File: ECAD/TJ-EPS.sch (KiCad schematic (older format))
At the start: 29 parts

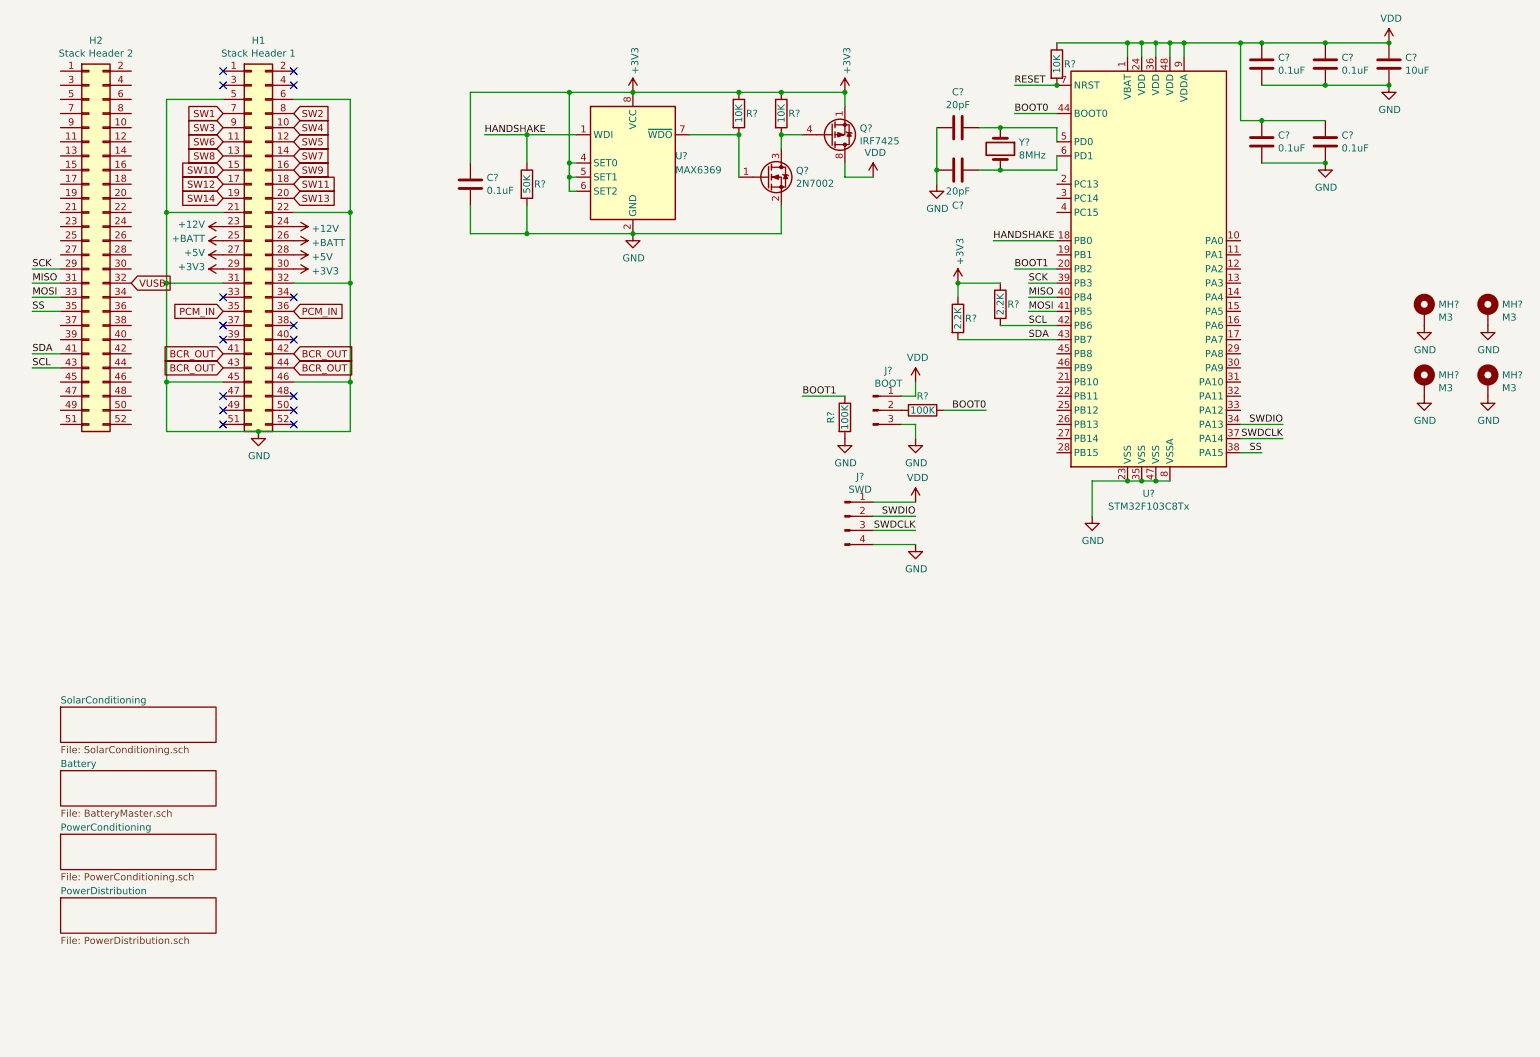
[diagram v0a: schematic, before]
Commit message: add amux
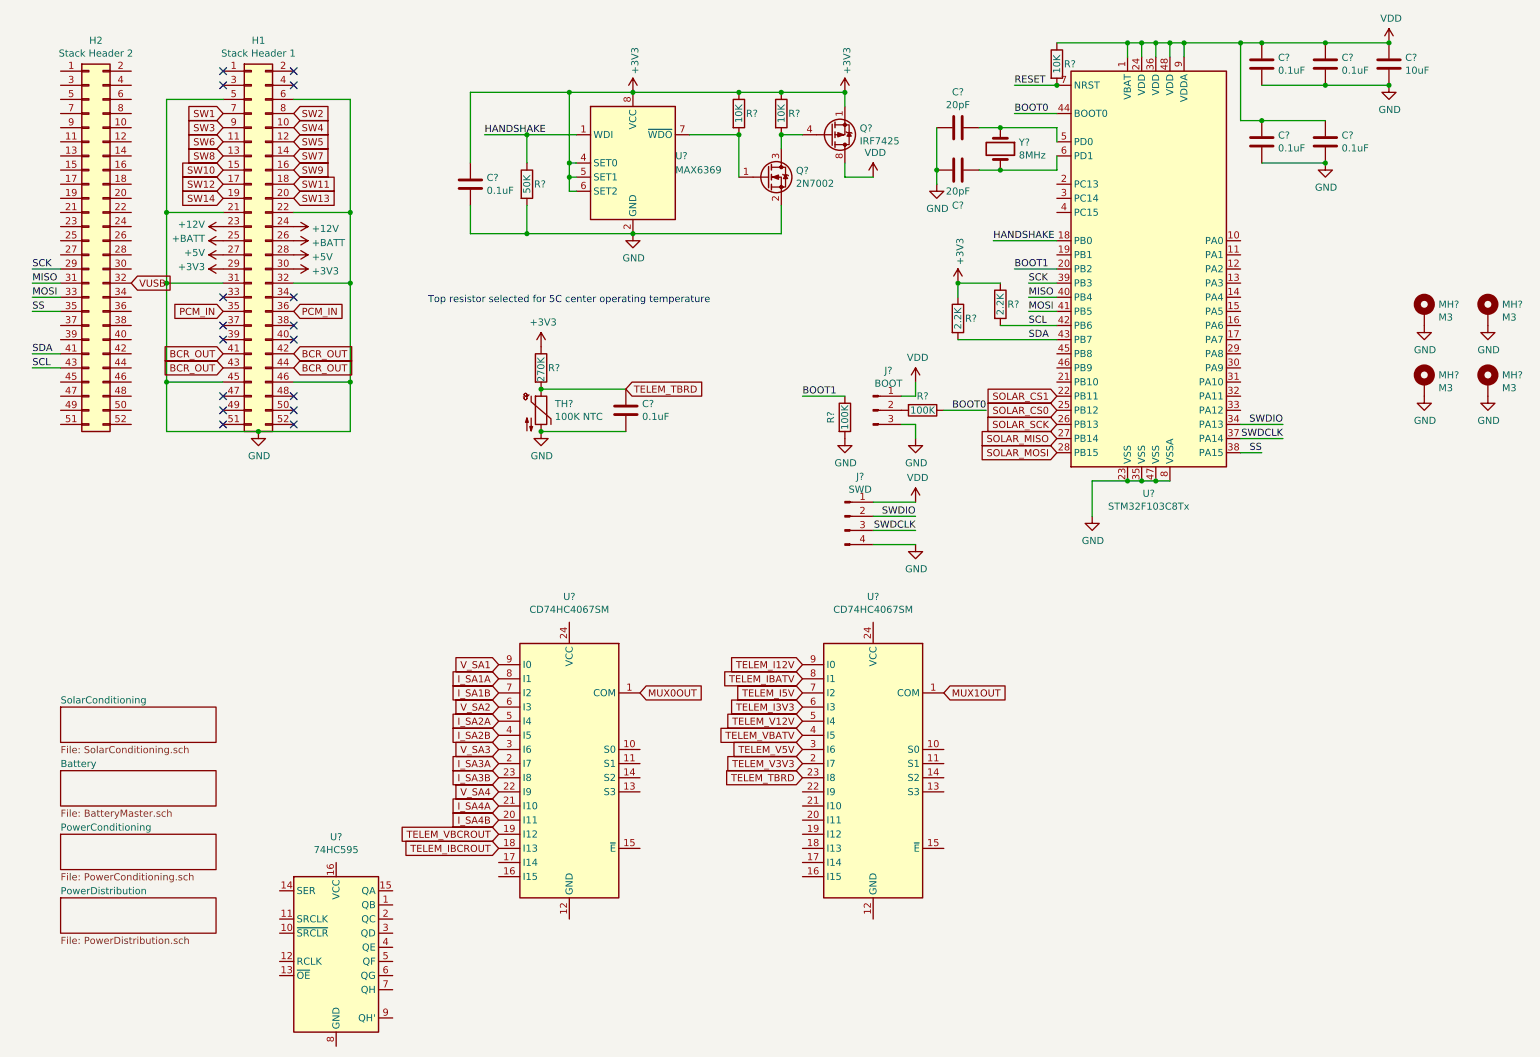
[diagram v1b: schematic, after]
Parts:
- added C?: 0.1uF, symbol Device:C
- added R?: 270K, symbol Device:R
- added TH?: 100K NTC, symbol Device:Thermistor_NTC
- added U? (x2): CD74HC4067SM, Package_SO:SSOP-24_5.3x8.2mm_P0.65mm, symbol 74xx:CD74HC4067SM
- added U?: 74HC595, symbol 74xx:74HC595
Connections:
- net +3V3: now also R?.1
- net GND: now also C?.2, TH?.2
- net SOLAR_CS1: now reaches U?.22 (PB11)
- net SOLAR_CS0: now reaches U?.25 (PB12)
- net SOLAR_SCK: now reaches U?.26 (PB13)
- net SOLAR_MISO: now reaches U?.27 (PB14)
- net SOLAR_MOSI: now reaches U?.28 (PB15)
- new net I_SA1A: U?.8 (I1)
- new net I_SA1B: U?.7 (I2)
- new net I_SA2A: U?.5 (I4)
- new net I_SA2B: U?.4 (I5)
- new net I_SA3A: U?.2 (I7)
- new net I_SA3B: U?.23 (I8)
- new net I_SA4A: U?.21 (I10)
- new net I_SA4B: U?.20 (I11)
- new net MUX0OUT: U?.1 (COM)
- new net MUX1OUT: U?.1 (COM)
- new net TELEM_I12V: U?.9 (I0)
- new net TELEM_I3V3: U?.6 (I3)
- new net TELEM_I5V: U?.7 (I2)
- new net TELEM_IBATV: U?.8 (I1)
- new net TELEM_IBCROUT: U?.18 (I13)
- new net TELEM_TBRD: C?.1, R?.2, TH?.1, U?.23 (I8)
- new net TELEM_V12V: U?.5 (I4)
- new net TELEM_V3V3: U?.2 (I7)
- new net TELEM_V5V: U?.3 (I6)
- new net TELEM_VBATV: U?.4 (I5)
- new net TELEM_VBCROUT: U?.19 (I12)
- new net V_SA1: U?.9 (I0)
- new net V_SA2: U?.6 (I3)
- new net V_SA3: U?.3 (I6)
- new net V_SA4: U?.22 (I9)
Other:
- note added: "Top resistor selected for 5C center operating temperature"
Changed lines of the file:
@@
 Wire Wire Line
 	550  3050 750  3050
+$Comp
+L 74xx:CD74HC4067SM U?
+U 1 1 61D924A0
+P 4350 5850
+F 0 "U?" H 4350 7031 50  0000 C CNN
+F 1 "CD74HC4067SM" H 4350 6940 50  0000 C CNN
+F 2 "Package_SO:SSOP-24_5.3x8.2mm_P0.65mm" H 5400 4850 50  0001 C CIN
+F 3 "http://www.ti.com/lit/ds/symlink/cd74hc4067.pdf" H 4000 6700 50  0001 C CNN
+	1    4350 5850
+	-1   0    0    -1
+$EndComp
+Text GLabel 3850 5250 0    50   Input ~ 0
+I_SA1A
+Text GLabel 3850 5550 0    50   Input ~ 0
+I_SA2A
+Text GLabel 3850 5650 0    50   Input ~ 0
+I_SA2B
+Text GLabel 3850 5850 0    50   Input ~ 0
+I_SA3A
+Text GLabel 3850 5950 0    50   Input ~ 0
+I_SA3B
+Text GLabel 3850 6150 0    50   Input ~ 0
+I_SA4A
+Text GLabel 3850 6250 0    50   Input ~ 0
+I_SA4B
+Text GLabel 3850 5350 0    50   Input ~ 0
+I_SA1B
+Text GLabel 3850 5150 0    50   Input ~ 0
+V_SA1
+Text GLabel 3850 5450 0    50   Input ~ 0
+V_SA2
+Text GLabel 3850 5750 0    50   Input ~ 0
+V_SA3
+Text GLabel 3850 6050 0    50   Input ~ 0
+V_SA4
+Text GLabel 3850 6350 0    50   Input ~ 0
+TELEM_VBCROUT
+Text GLabel 3850 6450 0    50   Input ~ 0
+TELEM_IBCROUT
+Text GLabel 6000 5150 0    50   Input ~ 0
+TELEM_I12V
+Text GLabel 6000 5250 0    50   Input ~ 0
+TELEM_IBATV
+Text GLabel 6000 5350 0    50   Input ~ 0
+TELEM_I5V
+Text GLabel 6000 5450 0    50   Input ~ 0
+TELEM_I3V3
+Text GLabel 6000 5550 0    50   Input ~ 0
+TELEM_V12V
+Text GLabel 6000 5650 0    50   Input ~ 0
+TELEM_VBATV
+Text GLabel 6000 5750 0    50   Input ~ 0
+TELEM_V5V
+Text GLabel 6000 5850 0    50   Input ~ 0
+TELEM_V3V3
+$Comp
+L Device:R R?
+U 1 1 6225F84D
+P 4150 3050
+AR Path="/61BD4B7D/62026259/6225F84D" Ref="R?"  Part="1"
+AR Path="/61BD4B7D/62041525/6225F84D" Ref="R?"  Part="1"
+AR Path="/61BD4B7D/62045EF1/6225F84D" Ref="R?"  Part="1"
+AR Path="/61BD4B7D/6204A8C5/6225F84D" Ref="R?"  Part="1"
+AR Path="/6225F84D" Ref="R?"  Part="1"
+F 0 "R?" H 4200 3050 50  0000 L CNN
+F 1 "270K" V 4150 2950 50  0000 L CNN
+F 2 "" V 4080 3050 50  0001 C CNN
+F 3 "~" H 4150 3050 50  0001 C CNN
+	1    4150 3050
+	1    0    0    -1
+$EndComp
+$Comp
+L Device:Thermistor_NTC TH?
+U 1 1 6225F853
+P 4150 3350
+AR Path="/61BD4B7D/62026259/6225F853" Ref="TH?"  Part="1"
+AR Path="/61BD4B7D/62041525/6225F853" Ref="TH?"  Part="1"
+AR Path="/61BD4B7D/62045EF1/6225F853" Ref="TH?"  Part="1"
+AR Path="/61BD4B7D/6204A8C5/6225F853" Ref="TH?"  Part="1"
+AR Path="/6225F853" Ref="TH?"  Part="1"
+F 0 "TH?" H 4248 3396 50  0000 L CNN
+F 1 "100K NTC" H 4248 3305 50  0000 L CNN
+F 2 "" H 4150 3400 50  0001 C CNN
+F 3 "~" H 4150 3400 50  0001 C CNN
+	1    4150 3350
+	1    0    0    -1
+$EndComp
+Text Notes 3350 2600 0    50   ~ 0
+Top resistor selected for 5C center operating temperature
+$Comp
+L power:+3V3 #PWR?
+U 1 1 6225F85A
+P 4150 2900
+AR Path="/61BD4B7D/62026259/6225F85A" Ref="#PWR?"  Part="1"
+AR Path="/61BD4B7D/62041525/6225F85A" Ref="#PWR?"  Part="1"
+AR Path="/61BD4B7D/62045EF1/6225F85A" Ref="#PWR?"  Part="1"
+AR Path="/61BD4B7D/6204A8C5/6225F85A" Ref="#PWR?"  Part="1"
+AR Path="/6225F85A" Ref="#PWR?"  Part="1"
+F 0 "#PWR?" H 4150 2750 50  0001 C CNN
+F 1 "+3V3" H 4165 3073 50  0000 C CNN
+F 2 "" H 4150 2900 50  0001 C CNN
+F 3 "" H 4150 2900 50  0001 C CNN
+	1    4150 2900
+	1    0    0    -1
+$EndComp
+Wire Wire Line
+	4150 3200 4750 3200
+Connection ~ 4150 3200
+$Comp
+L power:GND #PWR?
+U 1 1 6225F863
+P 4150 3500
+AR Path="/61BD4B7D/62026259/6225F863" Ref="#PWR?"  Part="1"
+AR Path="/61BD4B7D/62041525/6225F863" Ref="#PWR?"  Part="1"
+AR Path="/61BD4B7D/62045EF1/6225F863" Ref="#PWR?"  Part="1"
+AR Path="/61BD4B7D/6204A8C5/6225F863" Ref="#PWR?"  Part="1"
+AR Path="/6225F863" Ref="#PWR?"  Part="1"
+F 0 "#PWR?" H 4150 3250 50  0001 C CNN
+F 1 "GND" H 4155 3327 50  0000 C CNN
+F 2 "" H 4150 3500 50  0001 C CNN
+F 3 "" H 4150 3500 50  0001 C CNN
+	1    4150 3500
+	1    0    0    -1
+$EndComp
+Text GLabel 4750 3200 2    50   Input ~ 0
+TELEM_TBRD
+Connection ~ 4150 3500
+Wire Wire Line
+	4150 3500 4750 3500
+$Comp
+L Device:C C?
+U 1 1 6225F847
+P 4750 3350
+AR Path="/61BD4B7D/62026259/6225F847" Ref="C?"  Part="1"
+AR Path="/61BD4B7D/62041525/6225F847" Ref="C?"  Part="1"
+AR Path="/61BD4B7D/62045EF1/6225F847" Ref="C?"  Part="1"
+AR Path="/61BD4B7D/6204A8C5/6225F847" Ref="C?"  Part="1"
+AR Path="/6225F847" Ref="C?"  Part="1"
+F 0 "C?" H 4865 3396 50  0000 L CNN
+F 1 "0.1uF" H 4865 3305 50  0000 L CNN
+F 2 "" H 4788 3200 50  0001 C CNN
+F 3 "~" H 4750 3350 50  0001 C CNN
+	1    4750 3350
+	1    0    0    -1
+$EndComp
+$Comp
+L 74xx:CD74HC4067SM U?
+U 1 1 622718CA
+P 6500 5850
+F 0 "U?" H 6500 7031 50  0000 C CNN
+F 1 "CD74HC4067SM" H 6500 6940 50  0000 C CNN
+F 2 "Package_SO:SSOP-24_5.3x8.2mm_P0.65mm" H 7550 4850 50  0001 C CIN
+F 3 "http://www.ti.com/lit/ds/symlink/cd74hc4067.pdf" H 6150 6700 50  0001 C CNN
+	1    6500 5850
+	-1   0    0    -1
+$EndComp
+Text GLabel 6000 5950 0    50   Input ~ 0
+TELEM_TBRD
+Text GLabel 7800 3450 0    50   Input ~ 0
+SOLAR_SCK
+Text GLabel 7800 3550 0    50   Input ~ 0
+SOLAR_MISO
+Text GLabel 7800 3650 0    50   Input ~ 0
+SOLAR_MOSI
+Text GLabel 7800 3350 0    50   Input ~ 0
+SOLAR_CS0
+Text GLabel 7800 3250 0    50   Input ~ 0
+SOLAR_CS1
+Text GLabel 4850 5350 2    50   Input ~ 0
+MUX0OUT
+Text GLabel 7000 5350 2    50   Input ~ 0
+MUX1OUT
+$Comp
+L 74xx:74HC595 U?
+U 1 1 622B9EC0
+P 2700 7150
+F 0 "U?" H 2700 7931 50  0000 C CNN
+F 1 "74HC595" H 2700 7840 50  0000 C CNN
+F 2 "" H 2700 7150 50  0001 C CNN
+F 3 "http://www.ti.com/lit/ds/symlink/sn74hc595.pdf" H 2700 7150 50  0001 C CNN
+	1    2700 7150
+	1    0    0    -1
+$EndComp
 $EndSCHEMATC

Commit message: connect amux
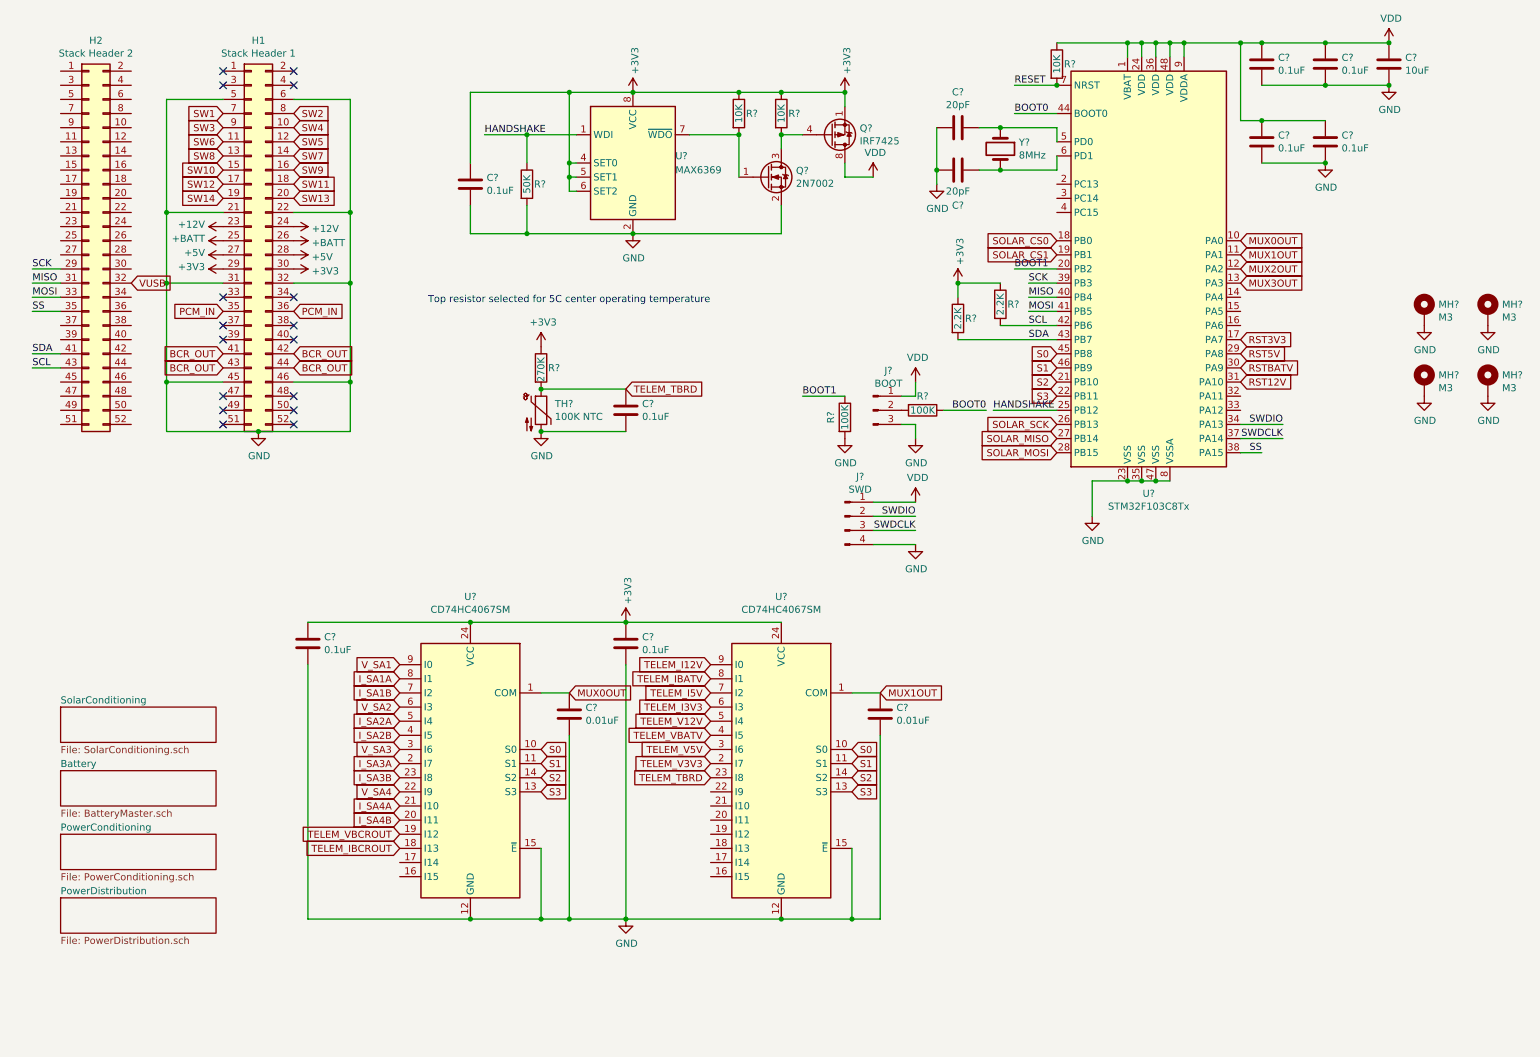
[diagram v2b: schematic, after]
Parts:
- removed U?: 74HC595, symbol 74xx:74HC595
- added C? (x2): 0.1uF, symbol Device:C
- added C? (x2): 0.01uF, symbol Device:C
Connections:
- net +3V3: now also U?.24 (VCC), U?.24 (VCC), C?.1, C?.1
- net GND: now also U?.12 (GND), U?.12 (GND), U?.15 (~E), U?.15 (~E), C?.2, C?.2, C?.2, C?.2
- net HANDSHAKE: now also U?.25 (PB12); no longer U?.18 (PB0)
- net MUX0OUT: now also U?.10 (PA0), C?.1
- net MUX1OUT: now also U?.11 (PA1), C?.1
- net SOLAR_CS0: now also U?.18 (PB0); no longer U?.25 (PB12)
- net SOLAR_CS1: now also U?.19 (PB1); no longer U?.22 (PB11)
- net S0: now reaches U?.10 (S0)
- net S0: now also U?.10 (S0), U?.45 (PB8)
- net S1: now reaches U?.11 (S1)
- net S1: now also U?.11 (S1), U?.46 (PB9)
- net S3: now reaches U?.13 (S3)
- net S3: now also U?.13 (S3), U?.22 (PB11)
- net S2: now reaches U?.14 (S2)
- net S2: now also U?.14 (S2), U?.21 (PB10)
- net MUX2OUT: now reaches U?.12 (PA2)
- net MUX3OUT: now reaches U?.13 (PA3)
- net RST3V3: now reaches U?.17 (PA7)
- net RST5V: now reaches U?.29 (PA8)
- net RSTBATV: now reaches U?.30 (PA9)
- net RST12V: now reaches U?.31 (PA10)
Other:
- moved on the sheet: U?

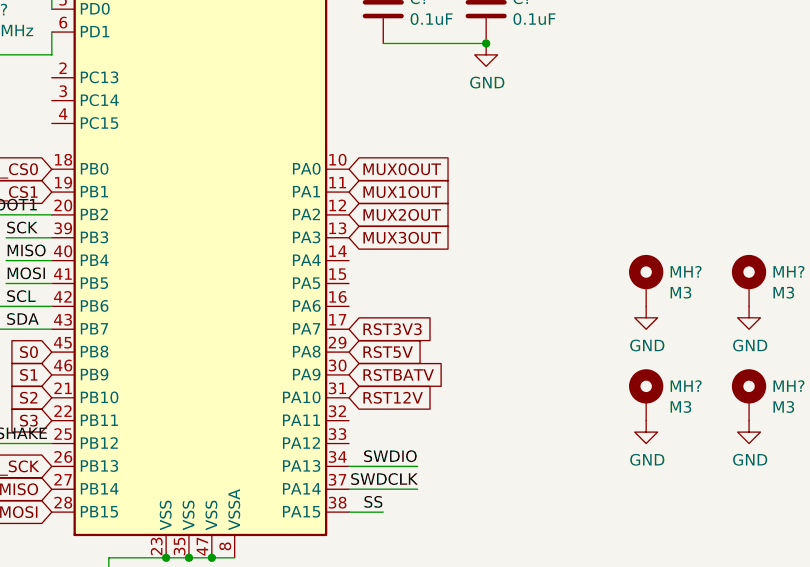
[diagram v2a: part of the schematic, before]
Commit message: Add PDM control using shift registers
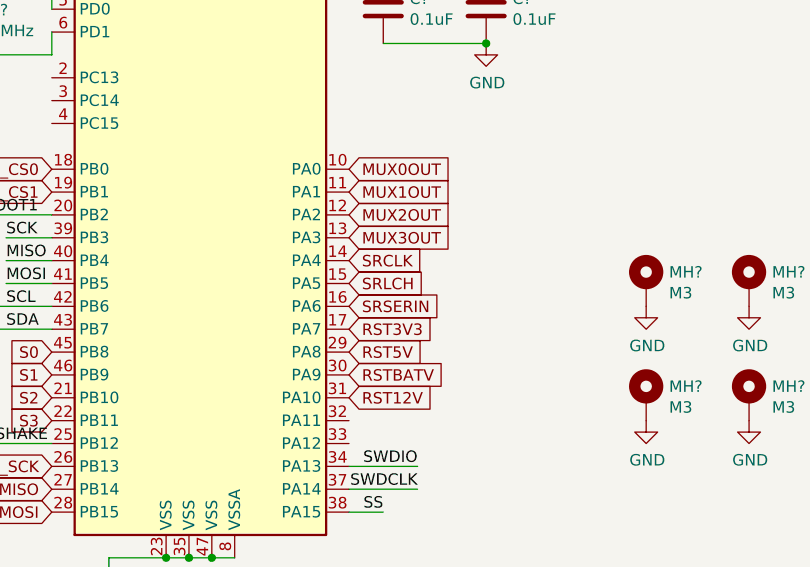
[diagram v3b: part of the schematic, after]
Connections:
- net SRCLK: now reaches U?.14 (PA4)
- net SRLCH: now reaches U?.15 (PA5)
- net SRSERIN: now reaches U?.16 (PA6)
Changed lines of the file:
@@
 Text GLabel 9100 2850 2    50   Input ~ 0
 RST3V3
+Text GLabel 9100 2550 2    50   Input ~ 0
+SRCLK
+Text GLabel 9100 2650 2    50   Input ~ 0
+SRLCH
+Text GLabel 9100 2750 2    50   Input ~ 0
+SRSERIN
 $EndSCHEMATC
